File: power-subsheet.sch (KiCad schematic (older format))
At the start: 0 parts

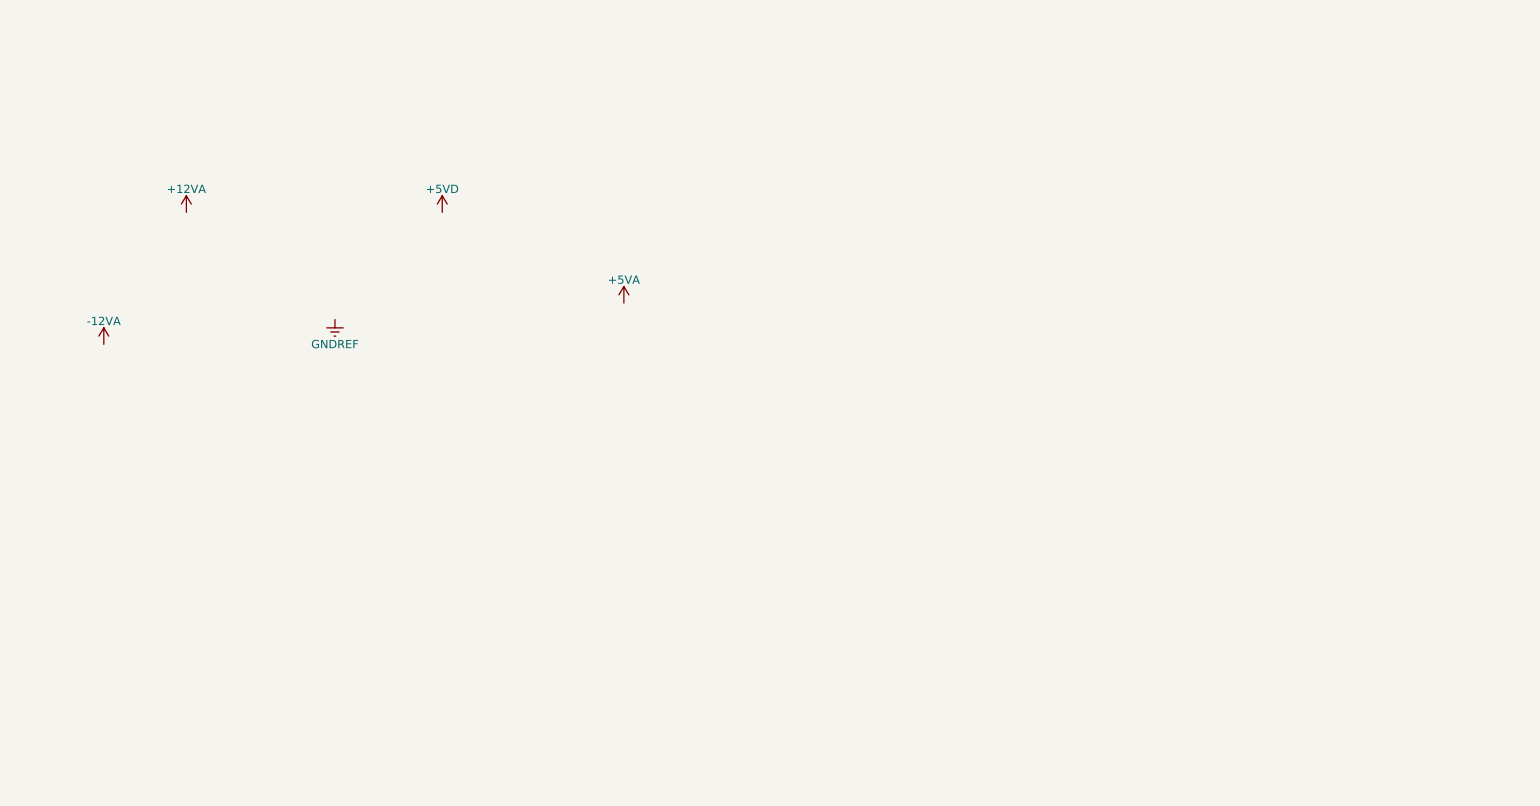
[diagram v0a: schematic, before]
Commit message: finished with first draft of schematic
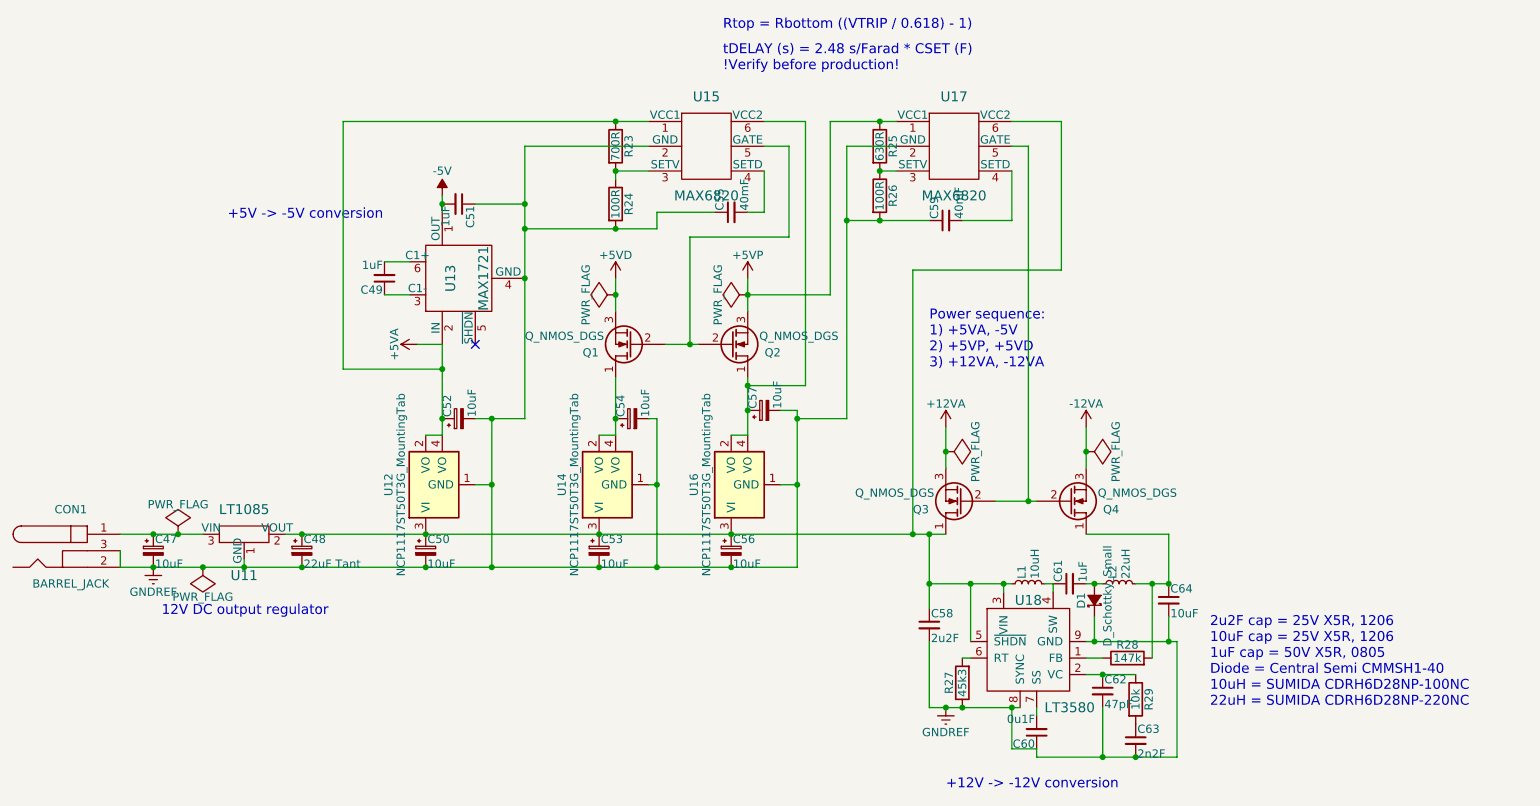
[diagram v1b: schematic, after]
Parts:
- added C47, C50, C52, C53, C54, C56, C57: 10uF, symbol CP_Small
- added C48: 22uF Tant, symbol CP_Small
- added C49, C51, C61: 1uF, symbol C_Small
- added C55, C59: 40mF, symbol C_Small
- added C58: 2u2F, symbol C_Small
- added C60: 0u1F, symbol C_Small
- added C62: 47pF, symbol C_Small
- added C63: 2n2F, symbol C_Small
- added C64: 10uF, symbol C_Small
- added CON1: BARREL_JACK, symbol BARREL_JACK
- added D1: D_Schottky_Small, symbol D_Schottky_Small
- added L1: 10uH, symbol L_Small
- added L2: 22uH, symbol L_Small
- added Q1, Q2, Q3, Q4: Q_NMOS_DGS, symbol Q_NMOS_DGS
- added R23: 700R, symbol R
- added R24, R26: 100R, symbol R
- added R25: 630R, symbol R
- added R27: 45k3, symbol R
- added R28: 147k, symbol R
- added R29: 10k, symbol R
- added U11: LT1085, symbol LT1085
- added U12, U14, U16: NCP1117ST50T3G_MountingTab, TO_SOT_Packages_SMD:SOT-223, symbol NCP1117ST50T3G_MountingTab
- added U13: MAX1721, symbol MAX1721
- added U15, U17: MAX6820, symbol MAX6820
- added U18: LT3580, symbol LT3580
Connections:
- net +12VA: now also Q3.3 (S)
- net +5VA: now also C52.1, R23.1, U12.2 (VO), U12.4 (VO), U13.2 (IN), U15.1 (VCC1)
- net +5VD: now also Q1.3 (S)
- net -12VA: now also Q4.3 (S)
- net GNDREF: now also C47.2, C48.2, C50.2, C51.1, C52.2, C53.2, C54.2, C55.1, C56.2, C57.2, C58.2, C59.1, C60.1, C62.2, C63.2, C64.2, CON1.2, CON1.3, D1.1 (K), R24.2, R26.2, R27.1, U11.1 (GND), U12.1 (GND), U13.4 (GND), U14.1 (GND), U15.2 (GND), U16.1 (GND), U17.2 (GND), U18.8 (SYNC), U18.9 (GND)
- new net: C48.1, C50.1, C53.1, C56.1, C58.1, L1.1, Q3.1 (D), U11.2 (VOUT), U12.3 (VI), U14.3 (VI), U16.3 (VI), U17.6 (VCC2), U18.3 (VIN), U18.5 (~SHDN)
- new net: C54.1, Q1.1 (D), U14.2 (VO), U14.4 (VO)
- new net: C57.1, Q2.1 (D), U15.6 (VCC2), U16.2 (VO), U16.4 (VO)
- new net: C47.1, CON1.1, U11.3 (VIN)
- new net: R25.2, R26.1, U17.3 (SETV)
- new net: C59.2, U17.4 (SETD)
- new net: Q3.2 (G), Q4.2 (G), U17.5 (GATE)
- new net: R23.2, R24.1, U15.3 (SETV)
- new net: C55.2, U15.4 (SETD)
- new net: Q1.2 (G), Q2.2 (G), U15.5 (GATE)
- new net: C49.1, U13.3 (C1-)
- new net: C49.2, U13.6 (C1+)
- new net: C64.1, L2.2, Q4.1 (D), R28.2
- new net: R28.1, U18.1 (FB)
- new net: C62.1, R29.1, U18.2 (VC)
- new net: C61.1, L1.2, U18.4 (SW)
- new net: R27.2, U18.6 (RT)
- new net: C60.2, U18.7 (SS)
- new net: C61.2, D1.2 (A), L2.1
- new net: C63.1, R29.2
- new net +5VP: Q2.3 (S), R25.1, U17.1 (VCC1)
- new net -5V: C51.2, U13.1 (OUT)
- no-connect marks 0 -> 1
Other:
- note added: "+12V -> -12V conversion"
- note added: "+5V -> -5V conversion"
- note added: "12V DC output regulator"
- note added: "2u2F cap = 25V X5R, 1206\n10uF cap = 25V X5R, 1206\n1uF cap = 50V X5R, 0805\nDiode = Central Semi CMMSH1-40\n10uH = SUMIDA CDRH6D28NP-100NC\n22uH = SUMIDA CDRH6D28NP-220NC"
- note added: "Power sequence:\n1) +5VA, -5V\n2) +5VP, +5VD\n3) +12VA, -12VA"
- note added: "Rtop = Rbottom ((VTRIP / 0.618) - 1) \n"
- note added: "tDELAY (s) = 2.48 s/Farad * CSET (F)\n!Verify before production!"
